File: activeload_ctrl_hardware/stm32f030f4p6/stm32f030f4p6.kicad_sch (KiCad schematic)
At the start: 43 parts

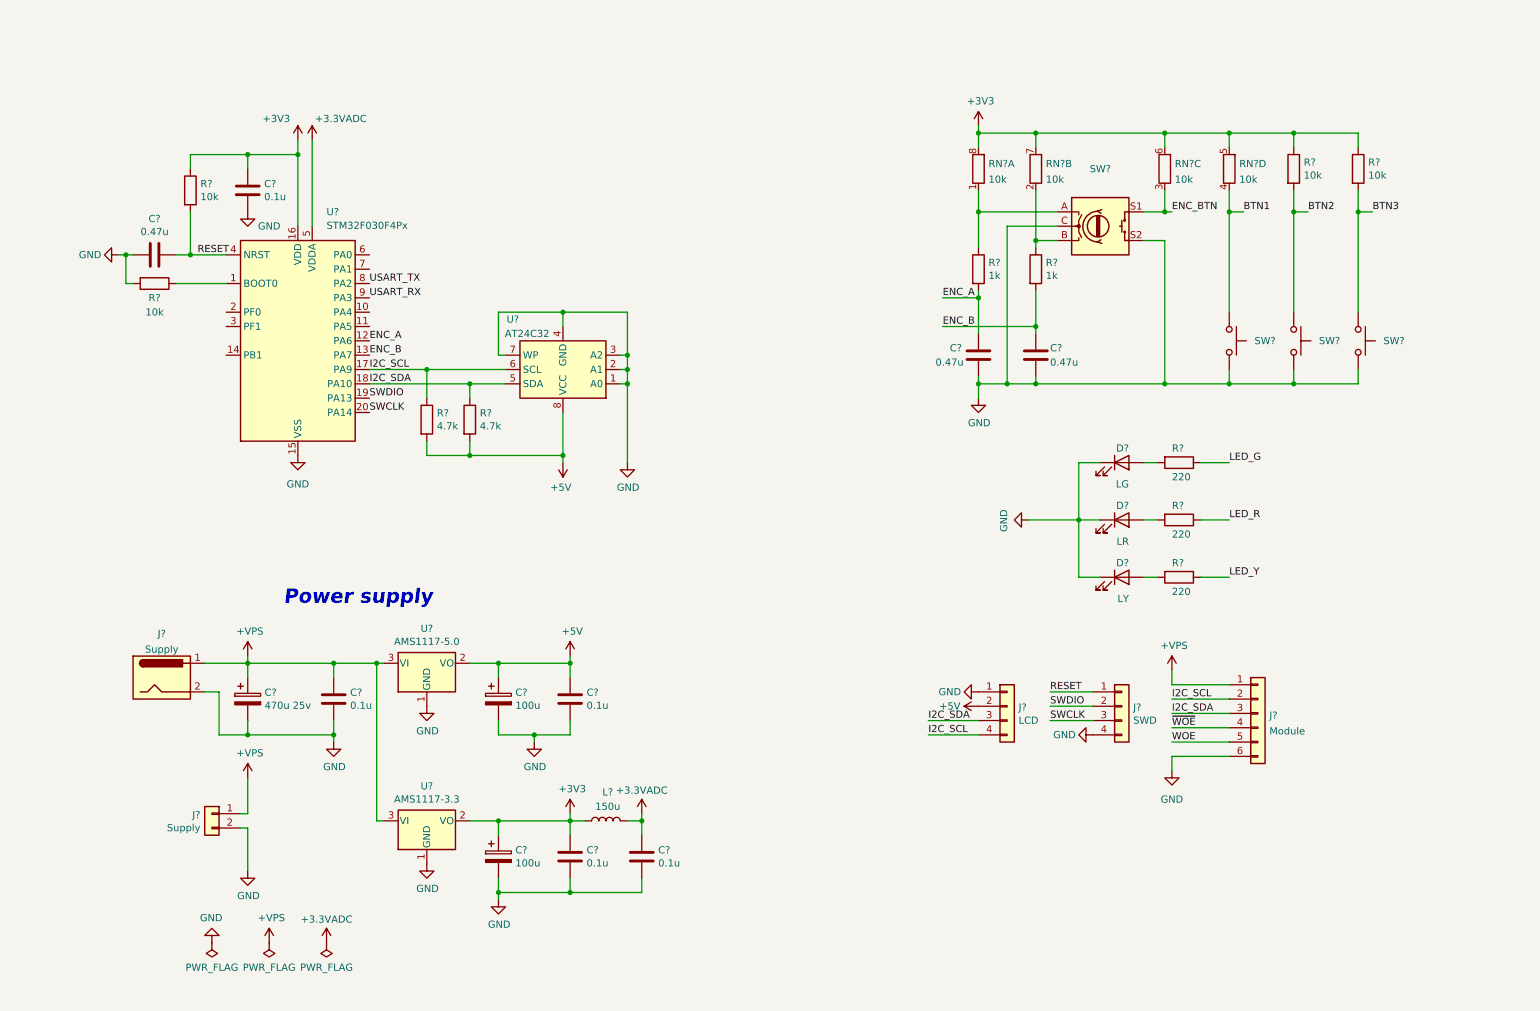
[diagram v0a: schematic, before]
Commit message: PCB start
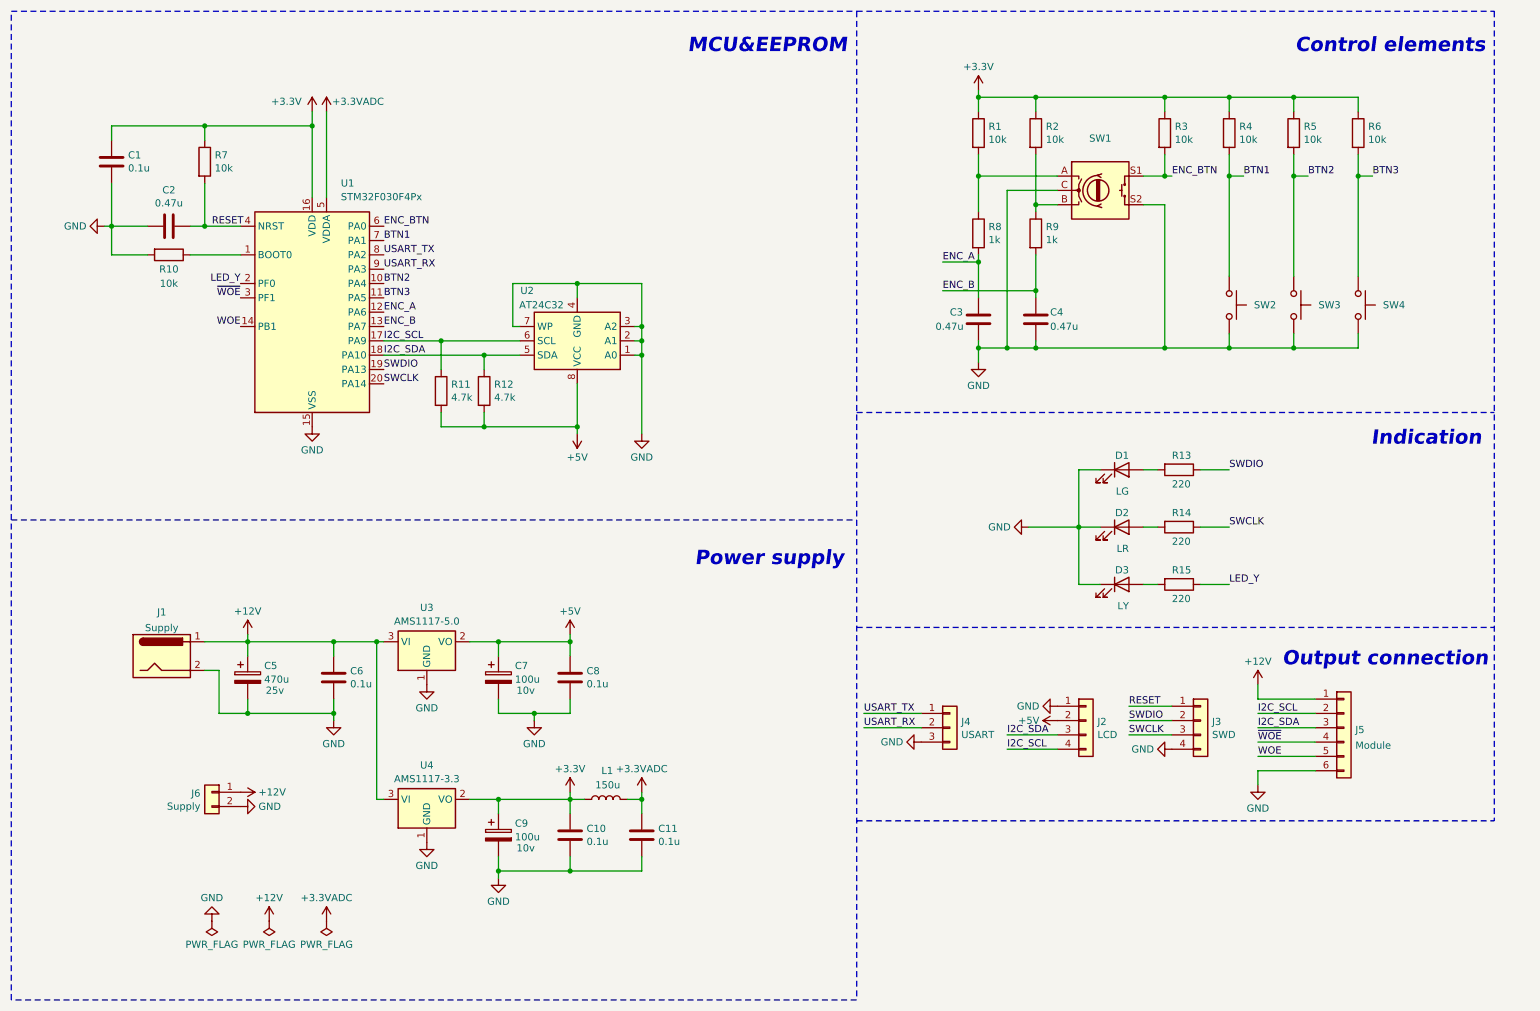
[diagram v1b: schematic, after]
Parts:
- removed C? (x2): 100u, Capacitor_THT:CP_Radial_D4.0mm_P2.00mm, symbol Device:CP
- removed C?: 470u 25v, Capacitor_THT:C_Radial_D8.0mm_H7.0mm_P3.50mm, symbol Device:CP
- removed R?: 10k, Resistor_SMD:R_1206_3216Metric_Pad1.30x1.75mm_HandSolder, symbol Device:R
- removed RN? (x4): 10k, Resistor_SMD:R_Array_Convex_4x1206, symbol Device:R_Pack04_Split
- removed SW?: (no value), Rotary_Encoder:RotaryEncoder_Alps_EC12E-Switch_Vertical_H20mm, symbol Device:Rotary_Encoder_Switch
- removed U?: AMS1117-5.0, Package_TO_SOT_SMD:SOT-223-3_TabPin2, symbol Regulator_Linear:AMS1117-5.0
- removed U?: AMS1117-3.3, Package_TO_SOT_SMD:SOT-223-3_TabPin2, symbol Regulator_Linear:AMS1117-3.3
- added C5: 470u, Capacitor_THT:C_Radial_D8.0mm_H7.0mm_P3.50mm, symbol Device:C_Polarized
- added C7, C9: 100u, Capacitor_THT:CP_Radial_D4.0mm_P2.00mm, symbol Device:C_Polarized
- added J4: USART, Connector_PinHeader_2.54mm:PinHeader_1x03_P2.54mm_Vertical, symbol Connector_Generic:Conn_01x03
- added R1, R2, R3, R4, R5: 10k, Resistor_SMD:R_1206_3216Metric_Pad1.30x1.75mm_HandSolder, symbol Device:R
- added SW1: ~, Rotary_Encoder:RotaryEncoder_Alps_EC12E-Switch_Vertical_H20mm, symbol Device:RotaryEncoder_Switch
- added U3: AMS1117-5.0, Package_TO_SOT_SMD:SOT-223-3_TabPin2, symbol Regulator_Linear:AMS1117-5.0
- added U4: AMS1117-3.3, Package_TO_SOT_SMD:SOT-223-3_TabPin2, symbol Regulator_Linear:AMS1117-3.3
- gave numbers to parts that had none: 32
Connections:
- net LED_G is gone; now on net SWDIO: R13.1
- net LED_R is gone; now on net SWCLK: R14.1
- net +5V: now also C7.1, U3.2 (VO)
- net BTN1: now also U1.7 (PA1), R4.2
- net BTN2: now also U1.10 (PA4), R5.2
- net BTN3: now also U1.11 (PA5)
- net ENC_BTN: now also U1.6 (PA0), R3.2, SW1.S1
- net GND: now also C5.2, C7.2, C9.2, J4.3 (Pin_3), SW1.C, SW1.S2, U3.1 (GND), U4.1 (GND)
- net LED_Y: now also U1.2 (PF0)
- net USART_RX: now also J4.2 (Pin_2)
- net USART_TX: now also J4.1 (Pin_1)
- net WOE: now also U1.14 (PB1)
- net ~{WOE}: now also U1.3 (PF1)
- net at R8.1: now also R1.2, SW1.A
- net at R9.1: now also R2.2, SW1.B
- net +3V3 renamed +3.3V
- net +3.3V: now also C9.1, R1.1, R2.1, R3.1, R4.1, R5.1, U4.2 (VO)
- net +VPS renamed +12V
- net +12V: now also C5.1, U3.3 (VI), U4.3 (VI)
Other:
- note added: "Control elements"
- note added: "Indication"
- note added: "MCU&EEPROM"
- note added: "Output connection"
- moved on the sheet: C1, C10, C11, C2, C3, C4, C6, C8, D1, D2, D3, J1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
